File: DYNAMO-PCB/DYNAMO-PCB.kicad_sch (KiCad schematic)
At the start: 14 parts, among them J13 Conn_01x02_Pin, J18 USB3_A, J20 HDMI_A, J21 USB3_A, J22 USB3_A, J23 USB3_A, J24 USB3_A, J25 USB3_A, J27 HDMI_A, J3 Conn_01x03_Pin, J34 Conn_02x05_Counter_Clockwise

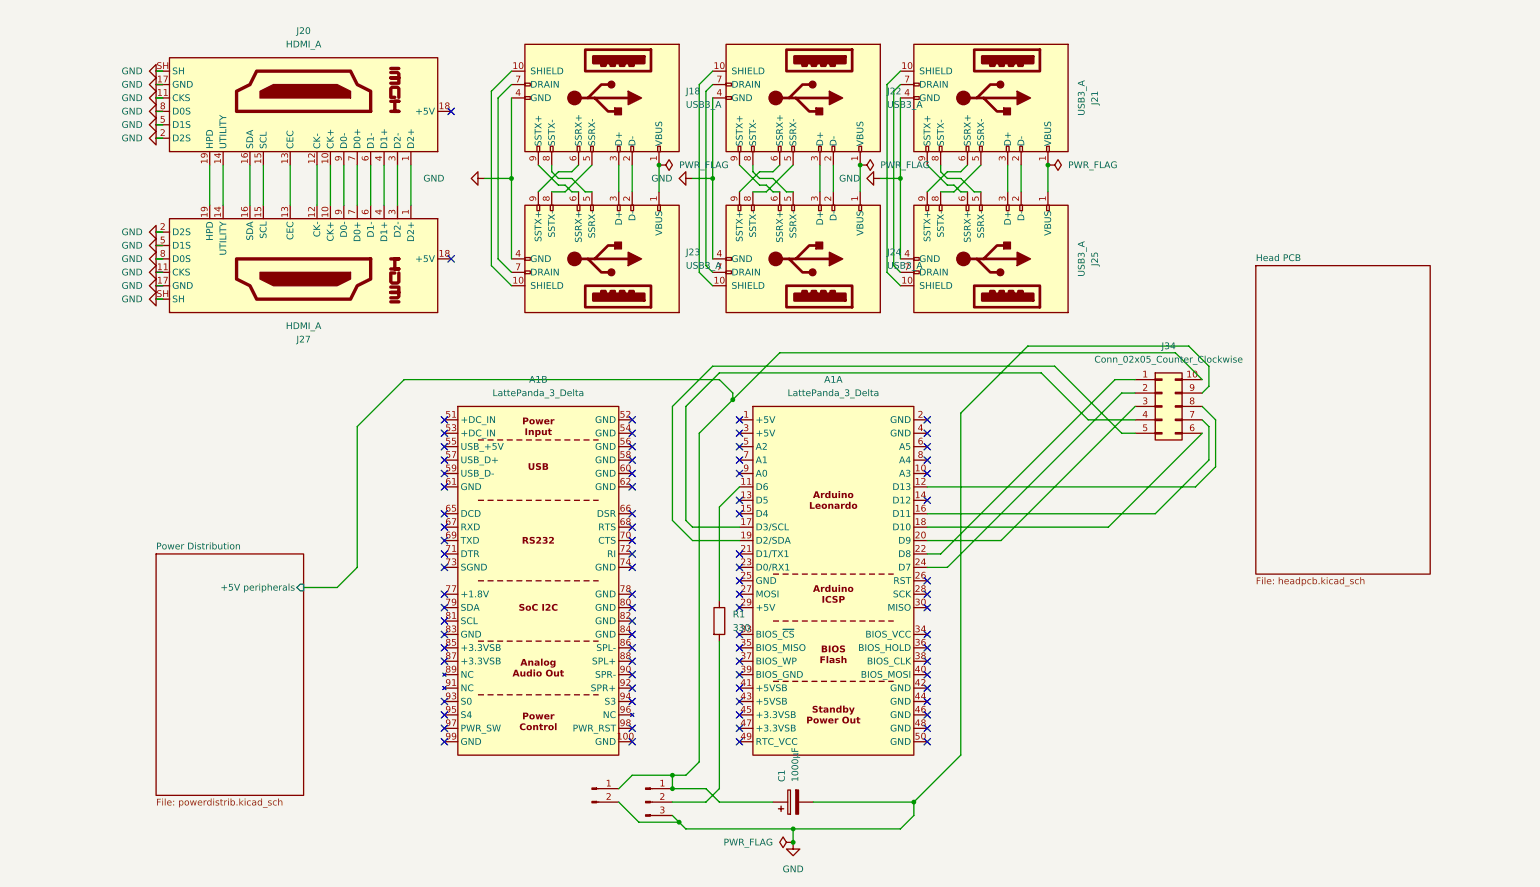
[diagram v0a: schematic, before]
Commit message: placement wip
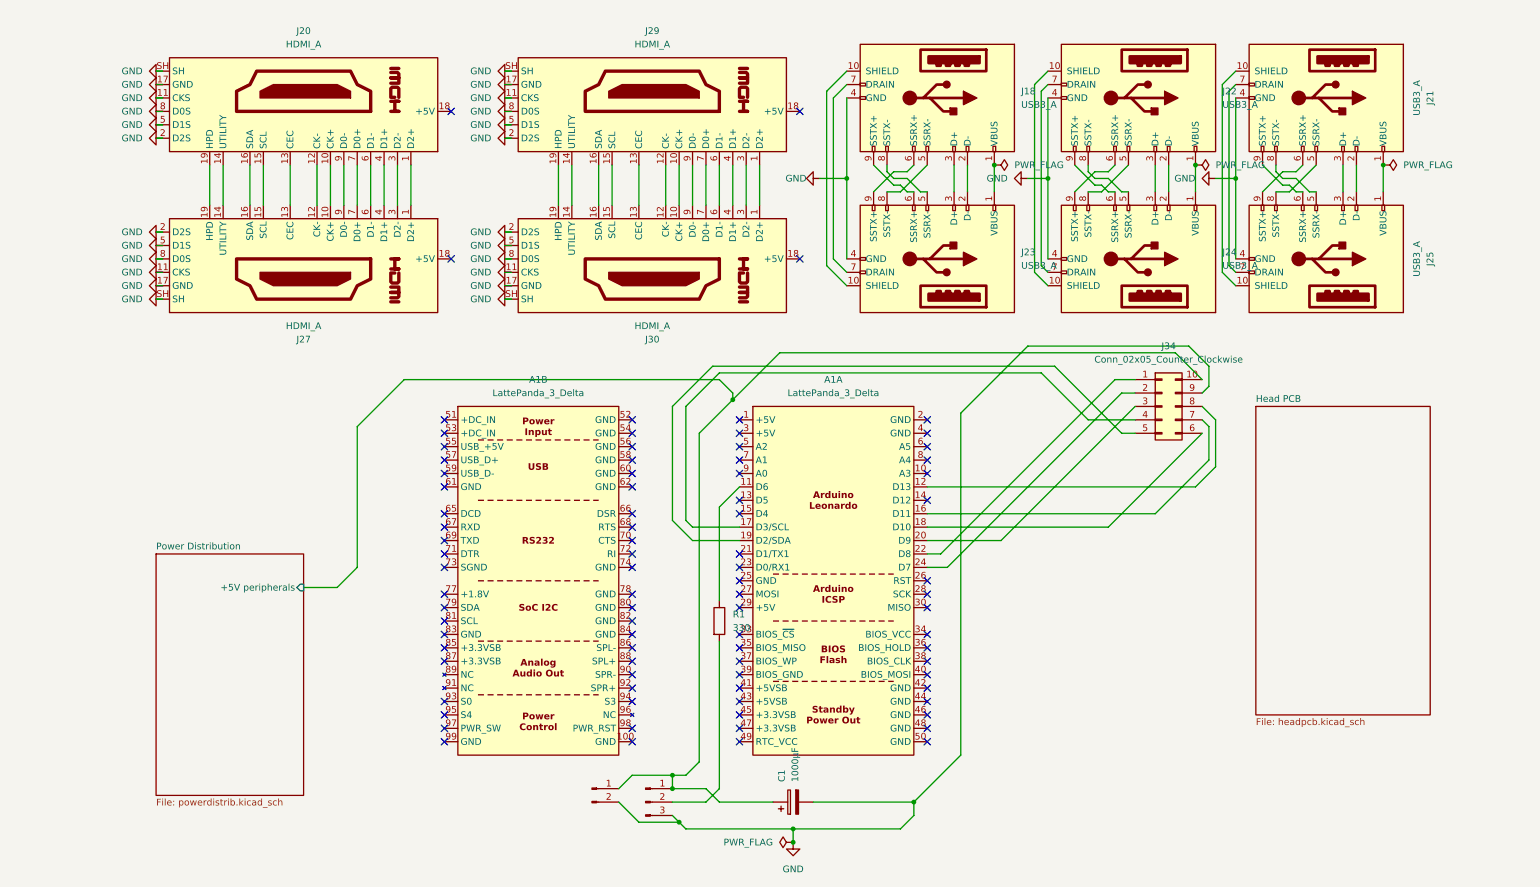
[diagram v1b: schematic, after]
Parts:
- added J29, J30: HDMI_A, Connector_Video:HDMI_A_Molex_208658-1001_Horizontal, symbol Connector:HDMI_A
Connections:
- net GND: now also J29.11 (CKS), J29.17 (GND), J29.2 (D2S), J29.5 (D1S), J29.8 (D0S), J29.SH, J30.11 (CKS), J30.17 (GND), J30.2 (D2S), J30.5 (D1S), J30.8 (D0S), J30.SH
- new net: J29.1 (D2+), J30.1 (D2+)
- new net: J29.10 (CK+), J30.10 (CK+)
- new net: J29.12 (CK-), J30.12 (CK-)
- new net: J29.13 (CEC), J30.13 (CEC)
- new net: J29.14 (UTILITY), J30.14 (UTILITY)
- new net: J29.15 (SCL), J30.15 (SCL)
- new net: J29.16 (SDA), J30.16 (SDA)
- new net: J29.19 (HPD), J30.19 (HPD)
- new net: J29.3 (D2-), J30.3 (D2-)
- new net: J29.4 (D1+), J30.4 (D1+)
- new net: J29.6 (D1-), J30.6 (D1-)
- new net: J29.7 (D0+), J30.7 (D0+)
- new net: J29.9 (D0-), J30.9 (D0-)
- no-connect marks 84 -> 86
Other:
- moved on the sheet: J18, J21, J22, J23, J24, J25

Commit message: headphone jack
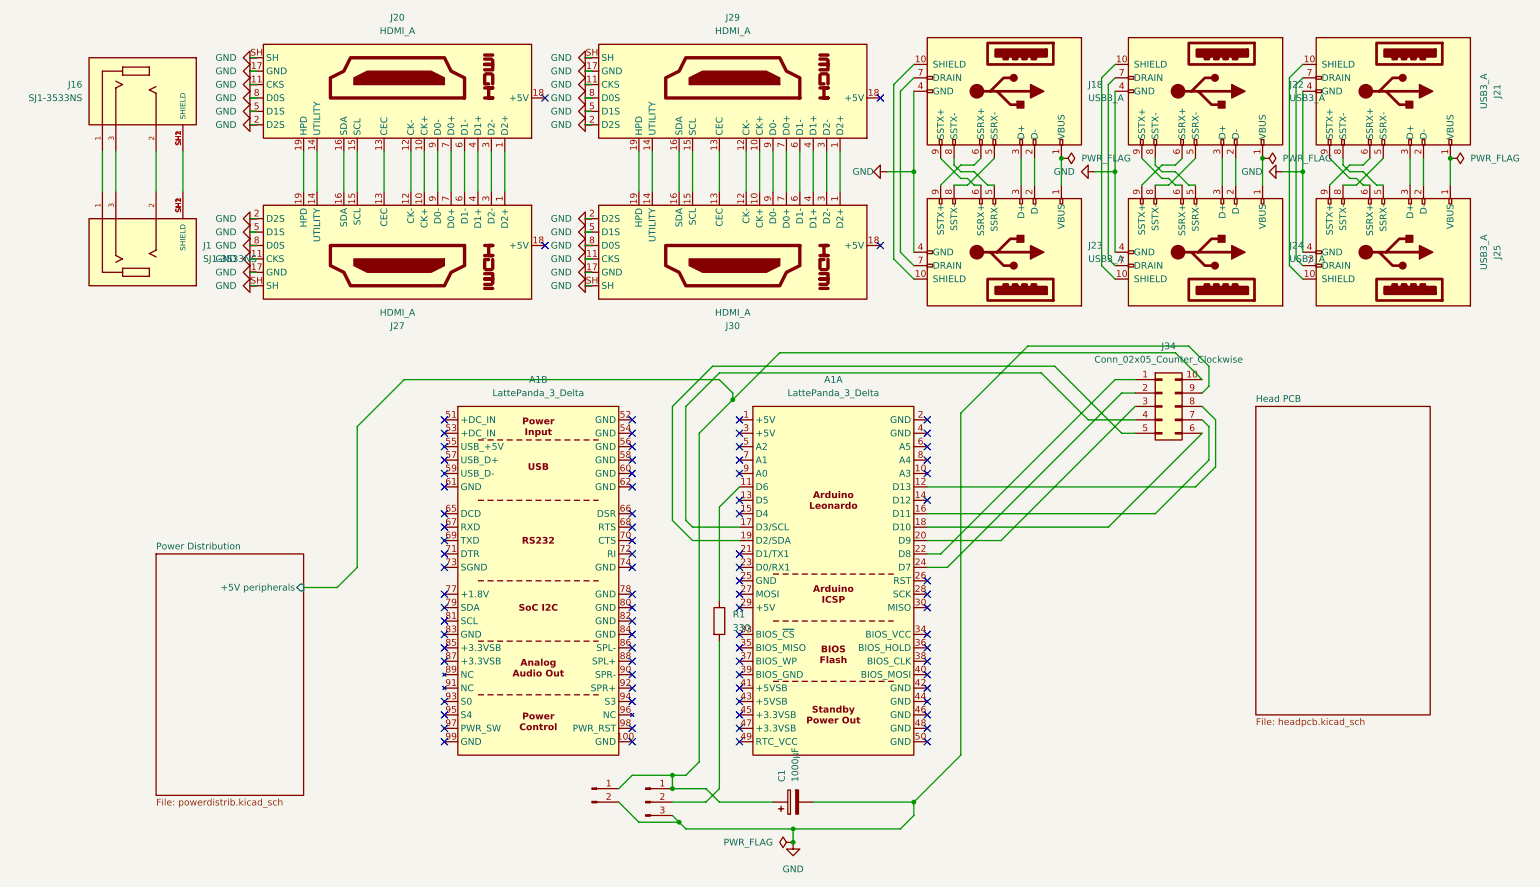
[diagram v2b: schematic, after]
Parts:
- added J1, J16: SJ1-3533NS, SJ1-3533NS:CUI_SJ1-3533NS, symbol SJ1-3533NS:SJ1-3533NS
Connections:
- new net: J1.1, J16.1
- new net: J1.2, J16.2
- new net: J1.3, J16.3
- new net: J1.SH1 (SHIELD), J1.SH2 (SHIELD), J1.SH3 (SHIELD), J16.SH1 (SHIELD), J16.SH2 (SHIELD), J16.SH3 (SHIELD)
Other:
- moved on the sheet: J18, J20, J21, J22, J23, J24, J25, J27, J29, J30

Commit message: routing
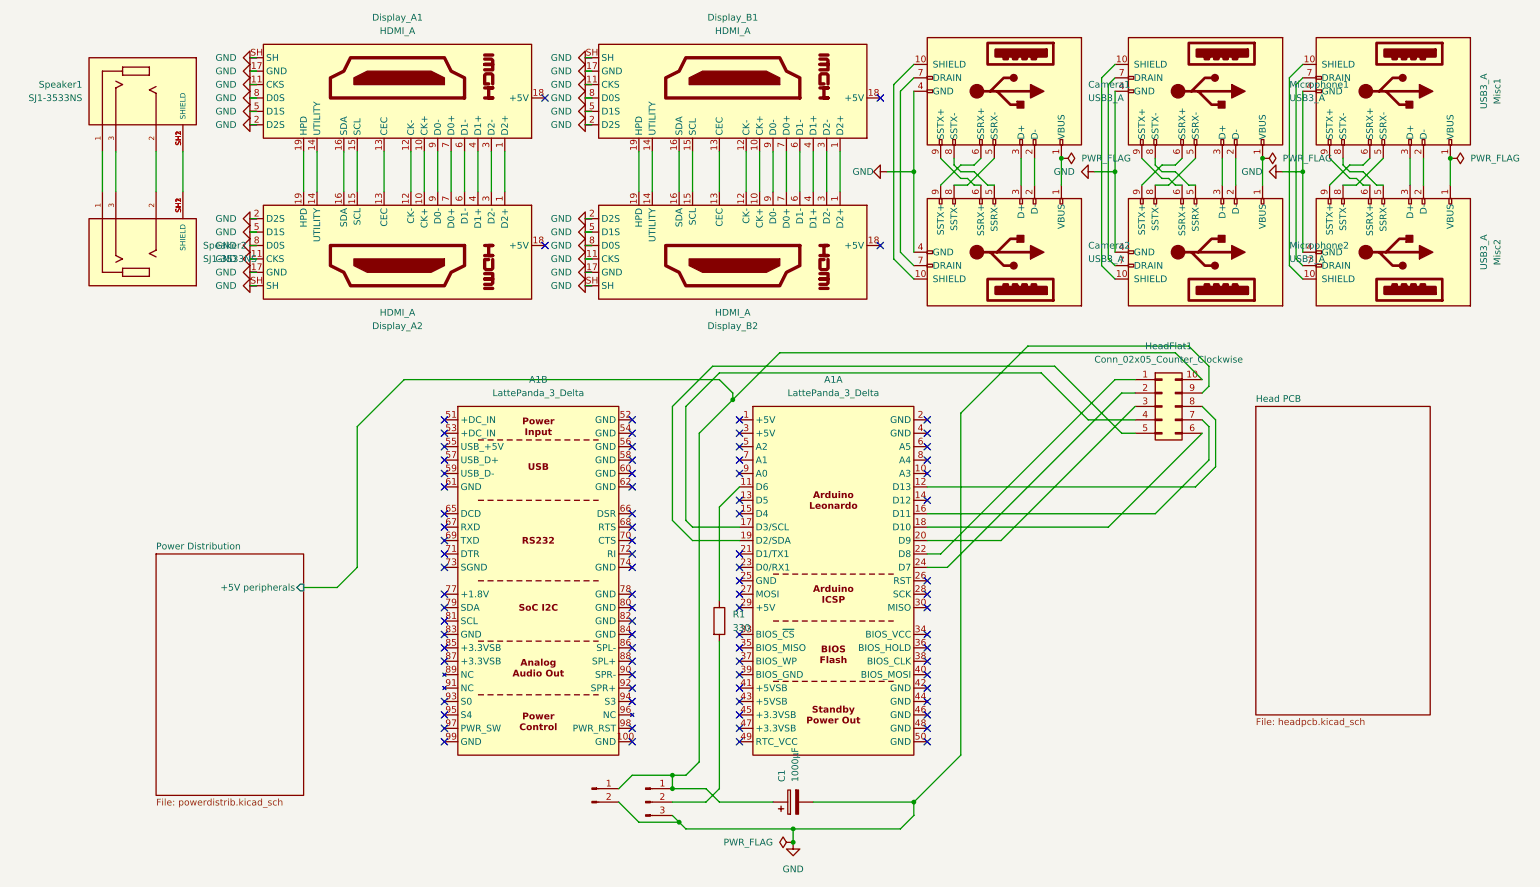
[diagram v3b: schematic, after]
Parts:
- renumbered J18 to Camera1, J23 to Camera2, J13 to CentralFan1, J3 to CentralLEDs1, J20 to Display_A1, J27 to Display_A2, J29 to Display_B1, J30 to Display_B2, J34 to HeadFlat1, J22 to Microphone1, J24 to Microphone2, J21 to Misc1, J25 to Misc2, J16 to Speaker1, J1 to Speaker2
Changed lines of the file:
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@@
 		(on_board yes)
 		(dnp no)
-		(property "Reference" "J24"
+		(property "Reference" "Microphone2"
 			(at 245.11 57.1499 90)
 			(effects
@@
 			(project "DYNAMO-PCB"
 				(path "/2ca9dd43-411d-4cc5-8a4b-ed00d72bae91"
-					(reference "J24")
+					(reference "Microphone2")
 					(unit 1)
 				)
@@
 		(on_board yes)
 		(dnp no)
-		(property "Reference" "J21"
+		(property "Reference" "Misc1"
 			(at 284.48 27.94 0)
 			(effects
@@
 			(project "DYNAMO-PCB"
 				(path "/2ca9dd43-411d-4cc5-8a4b-ed00d72bae91"
-					(reference "J21")
+					(reference "Misc1")
 					(unit 1)
 				)
@@
 		(on_board yes)
 		(dnp no)
-		(property "Reference" "J3"
+		(property "Reference" "CentralLEDs1"
 			(at 118.11 162.56 90)
 			(effects
@@
 			(project ""
 				(path "/2ca9dd43-411d-4cc5-8a4b-ed00d72bae91"
-					(reference "J3")
+					(reference "CentralLEDs1")
 					(unit 1)
 				)
@@
 		(on_board yes)
 		(dnp no)
-		(property "Reference" "J29"
+		(property "Reference" "Display_B1"
 			(at 139.7 13.97 90)
 			(effects
@@
 			(project "DYNAMO-PCB"
 				(path "/2ca9dd43-411d-4cc5-8a4b-ed00d72bae91"
-					(reference "J29")
+					(reference "Display_B1")
 					(unit 1)
 				)
@@
 		(on_board yes)
 		(dnp no)
-		(property "Reference" "J13"
+		(property "Reference" "CentralFan1"
 			(at 114.9351 163.83 90)
 			(effects
@@
 			(project "DYNAMO-PCB"
 				(path "/2ca9dd43-411d-4cc5-8a4b-ed00d72bae91"
-					(reference "J13")
+					(reference "CentralFan1")
 					(unit 1)
 				)
@@
 		(dnp no)
 		(fields_autoplaced yes)
-		(property "Reference" "J18"
+		(property "Reference" "Camera1"
 			(at 207.01 26.6699 90)
 			(effects
@@
 			(project "DYNAMO-PCB"
 				(path "/2ca9dd43-411d-4cc5-8a4b-ed00d72bae91"
-					(reference "J18")
+					(reference "Camera1")
 					(unit 1)
 				)
@@
 		(on_board yes)
 		(dnp no)
-		(property "Reference" "J25"
+		(property "Reference" "Misc2"
 			(at 284.48 58.42 0)
 			(effects
@@
 			(project "DYNAMO-PCB"
 				(path "/2ca9dd43-411d-4cc5-8a4b-ed00d72bae91"
-					(reference "J25")
+					(reference "Misc2")
 					(unit 1)
 				)
@@
 		(dnp no)
 		(fields_autoplaced yes)
-		(property "Reference" "J34"
+		(property "Reference" "HeadFlat1"
 			(at 222.25 76.2 0)
 			(effects
@@
 			(project "DYNAMO-PCB"
 				(path "/2ca9dd43-411d-4cc5-8a4b-ed00d72bae91"
-					(reference "J34")
+					(reference "HeadFlat1")
 					(unit 1)
 				)
@@
 		(on_board yes)
 		(dnp no)
-		(property "Reference" "J16"
+		(property "Reference" "Speaker1"
 			(at 16.51 26.6699 90)
 			(effects
@@
 			(project ""
 				(path "/2ca9dd43-411d-4cc5-8a4b-ed00d72bae91"
-					(reference "J16")
+					(reference "Speaker1")
 					(unit 1)
 				)
@@
 		(dnp no)
 		(fields_autoplaced yes)
-		(property "Reference" "J1"
+		(property "Reference" "Speaker2"
 			(at 39.37 57.1499 90)
 			(effects
@@
 			(project ""
 				(path "/2ca9dd43-411d-4cc5-8a4b-ed00d72bae91"
-					(reference "J1")
+					(reference "Speaker2")
 					(unit 1)
 				)
@@
 		(on_board yes)
 		(dnp no)
-		(property "Reference" "J30"
+		(property "Reference" "Display_B2"
 			(at 139.7 72.39 90)
 			(effects
@@
 			(project "DYNAMO-PCB"
 				(path "/2ca9dd43-411d-4cc5-8a4b-ed00d72bae91"
-					(reference "J30")
+					(reference "Display_B2")
 					(unit 1)
 				)
@@
 		(on_board yes)
 		(dnp no)
-		(property "Reference" "J27"
+		(property "Reference" "Display_A2"
 			(at 76.2 72.39 90)
 			(effects
@@
 			(project "DYNAMO-PCB"
 				(path "/2ca9dd43-411d-4cc5-8a4b-ed00d72bae91"
-					(reference "J27")
+					(reference "Display_A2")
 					(unit 1)
 				)
@@
 		(on_board yes)
 		(dnp no)
-		(property "Reference" "J23"
+		(property "Reference" "Camera2"
 			(at 207.01 57.1499 90)
 			(effects
@@
 			(project "DYNAMO-PCB"
 				(path "/2ca9dd43-411d-4cc5-8a4b-ed00d72bae91"
-					(reference "J23")
+					(reference "Camera2")
 					(unit 1)
 				)
@@
 		(on_board yes)
 		(dnp no)
-		(property "Reference" "J22"
+		(property "Reference" "Microphone1"
 			(at 245.11 26.6699 90)
 			(effects
@@
 			(project "DYNAMO-PCB"
 				(path "/2ca9dd43-411d-4cc5-8a4b-ed00d72bae91"
-					(reference "J22")
+					(reference "Microphone1")
 					(unit 1)
 				)
@@
 		(on_board yes)
 		(dnp no)
-		(property "Reference" "J20"
+		(property "Reference" "Display_A1"
 			(at 76.2 13.97 90)
 			(effects
@@
 			(project "DYNAMO-PCB"
 				(path "/2ca9dd43-411d-4cc5-8a4b-ed00d72bae91"
-					(reference "J20")
+					(reference "Display_A1")
 					(unit 1)
 				)
